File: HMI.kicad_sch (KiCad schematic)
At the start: 1 part, among them U8 XIAO-RP2350-SMD

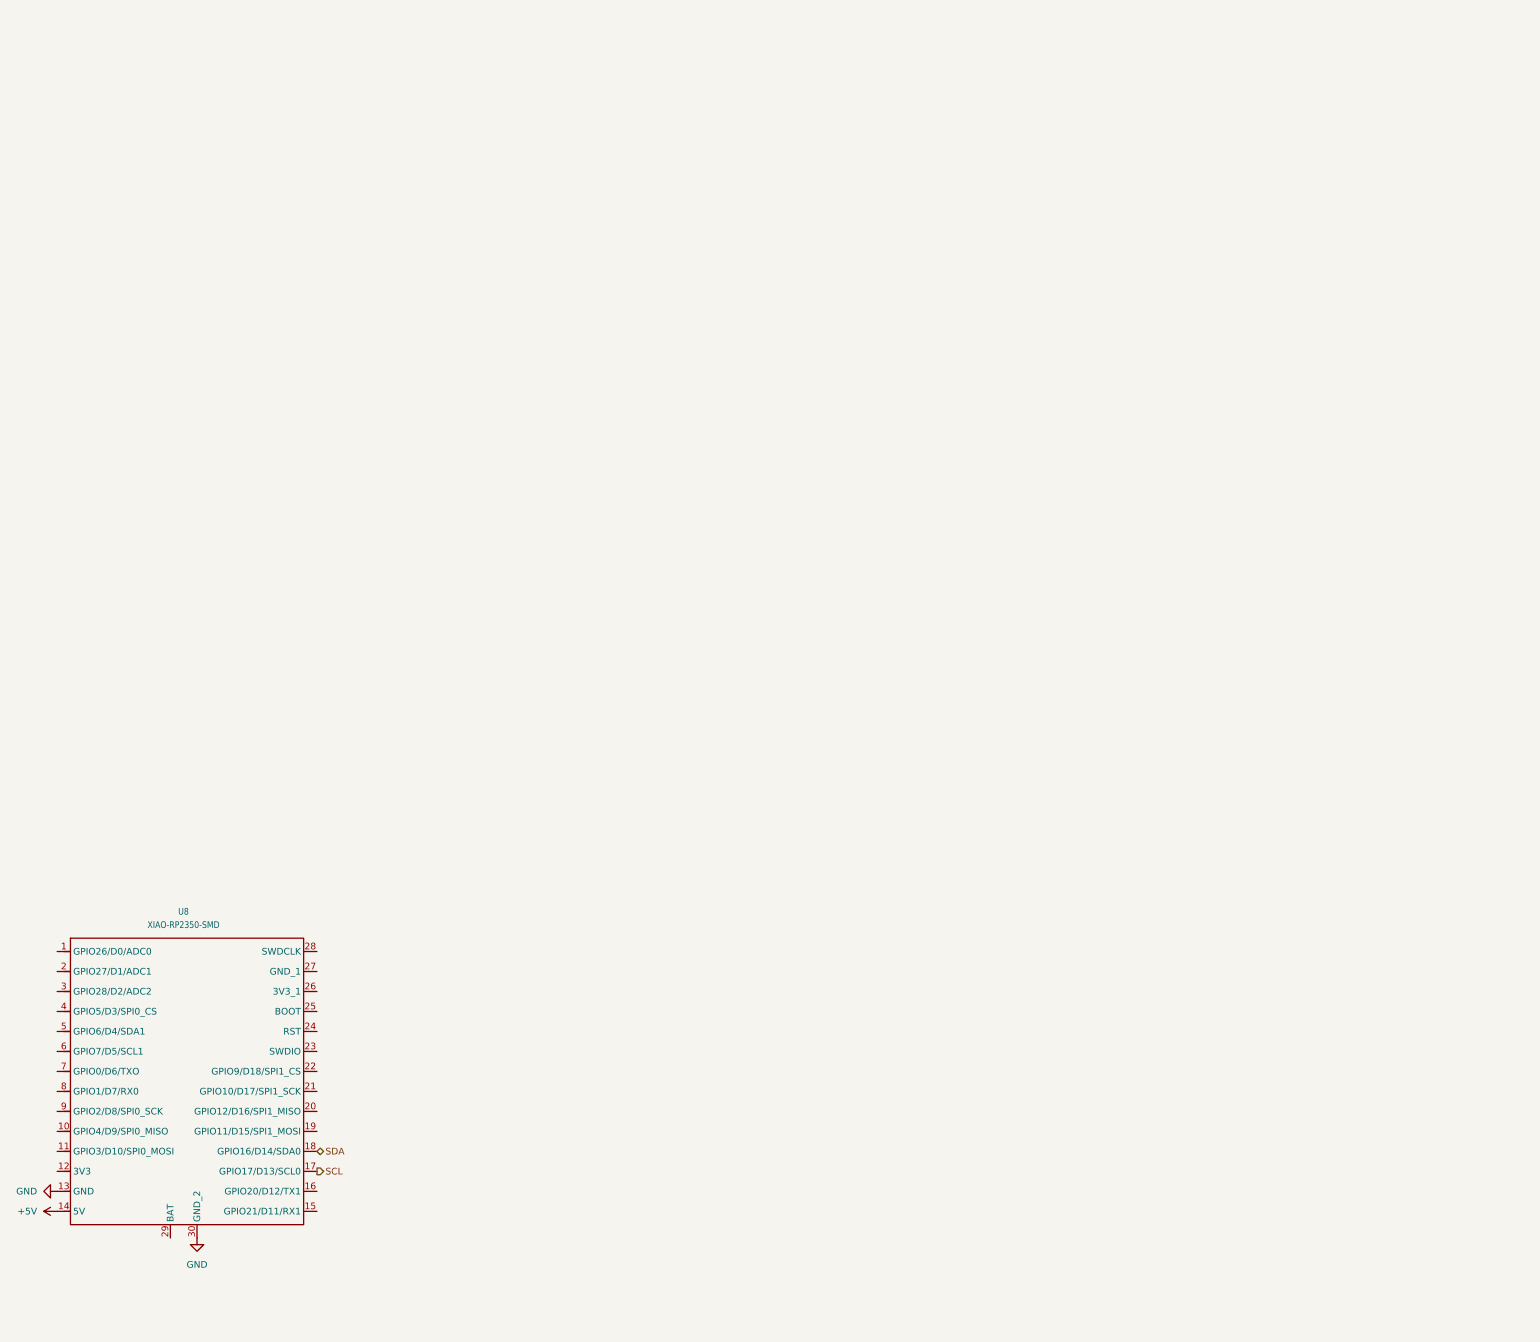
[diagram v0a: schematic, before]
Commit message: many changes
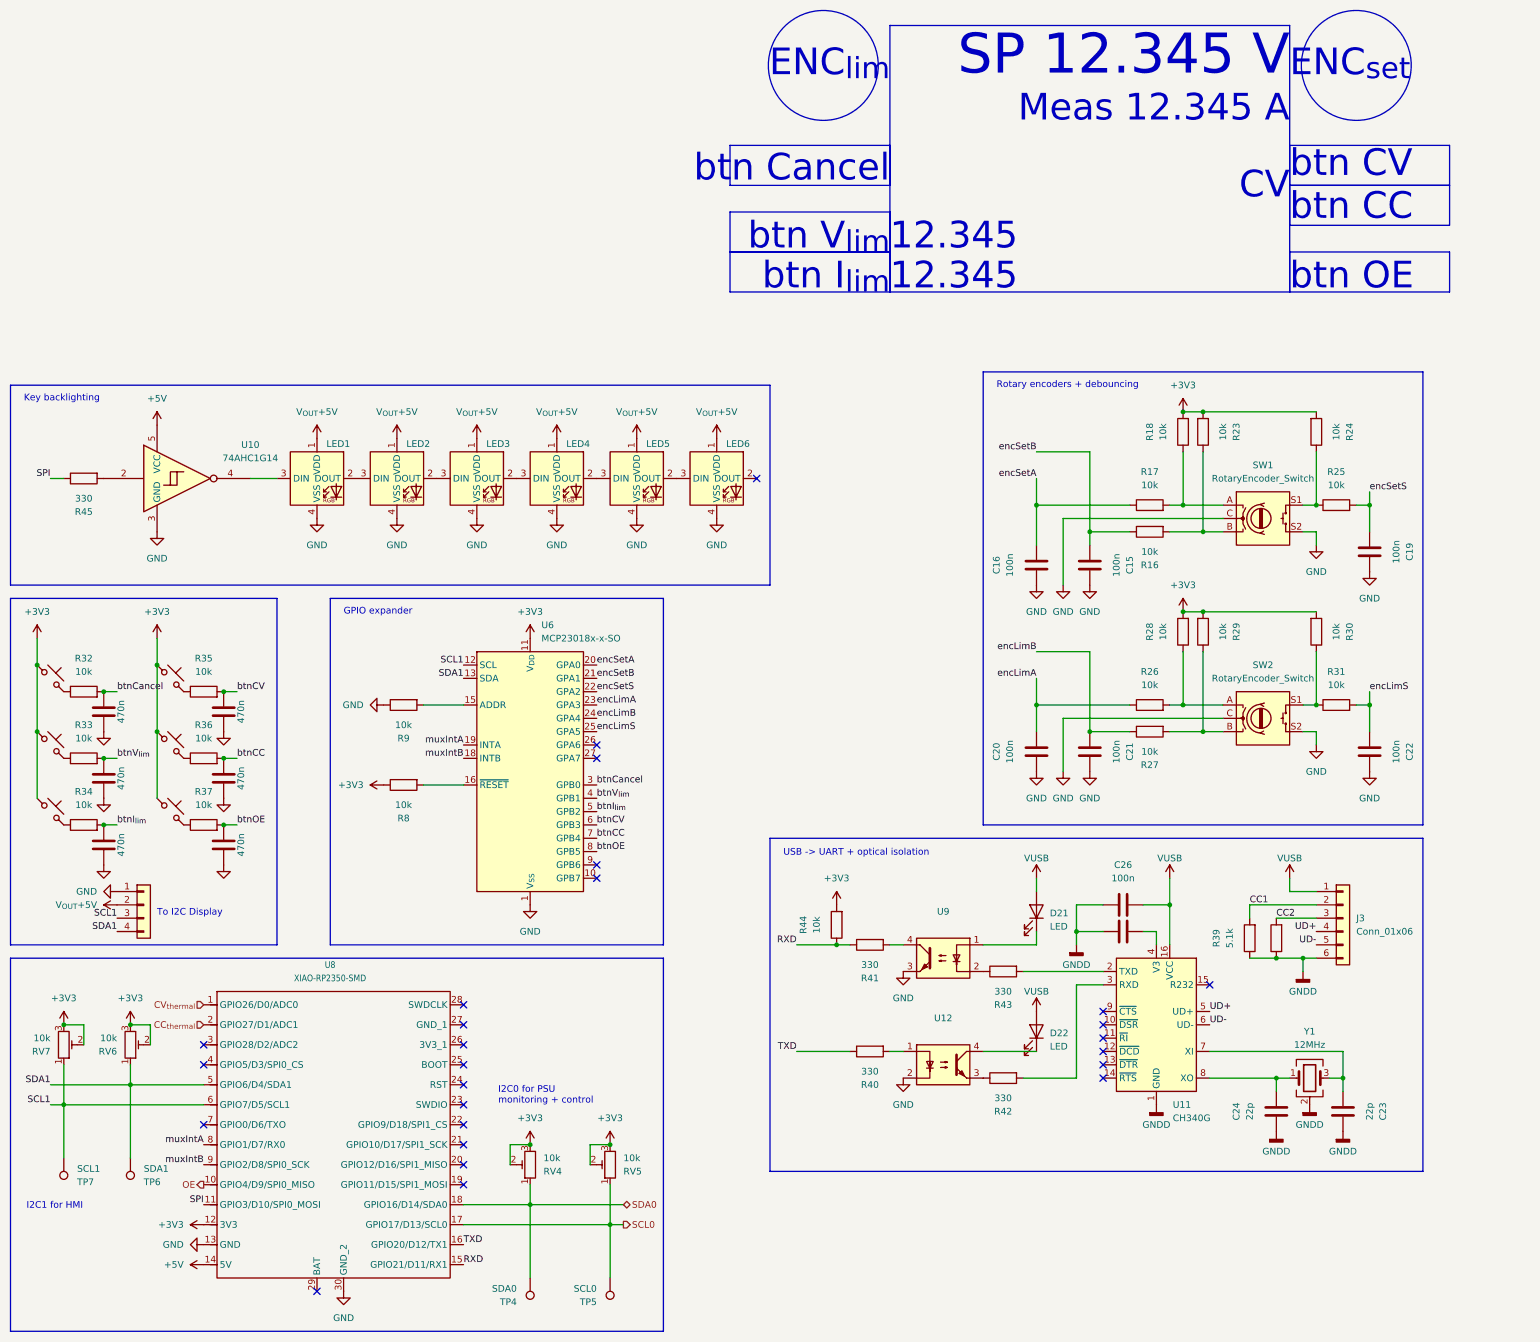
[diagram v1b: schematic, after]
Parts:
- added C12, C40, C41, C42, C43, C44: 470n, Capacitor_SMD:C_1210_3225Metric_Pad1.33x2.70mm_HandSolder, symbol Device:C
- added C15, C16, C19, C20, C21, C22, C25, C26: 100n, Capacitor_SMD:C_1210_3225Metric_Pad1.33x2.70mm_HandSolder, symbol Device:C
- added C23, C24: 22p, Capacitor_SMD:C_1210_3225Metric_Pad1.33x2.70mm_HandSolder, symbol Device:C
- added D21, D22: LED, LED_SMD:LED_1210_3225Metric_Pad1.42x2.65mm_HandSolder, symbol Device:LED
- added J2: Conn_01x04, I2C OLED:I2C OLED, symbol Connector_Generic:Conn_01x04
- added J3: Conn_01x06, Connector_JST:JST_PH_B6B-PH-K_1x06_P2.00mm_Vertical, symbol Connector_Generic:Conn_01x06
- added LED1, LED2, LED3, LED4, LED5, LED6: SK6812MINI-E, PCM_marbastlib-various:LED_6028R, symbol PCM_marbastlib-various:SK6812MINI-E
- added MX1, MX2, MX3, MX4, MX5, MX6: MX_SW_solder, PCM_marbastlib-mx:SW_MX_1u, symbol PCM_marbastlib-mx:MX_SW_solder
- added R16, R17, R18, R23, R24, R25, R26, R27, R28, R29, R30, R31, R32, R33, R34, R35, R36, R37, R44, R8, R9: 10k, Resistor_SMD:R_1210_3225Metric_Pad1.30x2.65mm_HandSolder, symbol Device:R
- added R38, R39: 5.1k, Resistor_SMD:R_1210_3225Metric_Pad1.30x2.65mm_HandSolder, symbol Device:R
- added R40, R41, R42, R43, R45: 330, Resistor_SMD:R_1210_3225Metric_Pad1.30x2.65mm_HandSolder, symbol Device:R
- added RV4, RV5, RV6, RV7: 10k, Potentiometer_THT:Potentiometer_Bourns_3299W_Vertical, symbol Device:R_Potentiometer_Trim
- added SW1, SW2: RotaryEncoder_Switch, Rotary_Encoder:RotaryEncoder_Alps_EC11E-Switch_Vertical_H20mm, symbol Device:RotaryEncoder_Switch
- added TP4: SDA0, TestPoint:TestPoint_Keystone_5019_Miniature, symbol Connector:TestPoint
- added TP5: SCL0, TestPoint:TestPoint_Keystone_5019_Miniature, symbol Connector:TestPoint
- added TP6: SDA1, TestPoint:TestPoint_Keystone_5019_Miniature, symbol Connector:TestPoint
- added TP7: SCL1, TestPoint:TestPoint_Keystone_5019_Miniature, symbol Connector:TestPoint
- added U10: 74AHC1G14, symbol 74xGxx:74AHC1G14
- added U11: CH340G, Package_SO:SOIC-16_3.9x9.9mm_P1.27mm, symbol Interface_USB:CH340G
- added U12, U9: Optocoupler_DC_PhotoNPN_AKEC, Package_DIP:DIP-4_W7.62mm_Socket_LongPads, symbol Isolator:Optocoupler_DC_PhotoNPN_AKEC
- added U6: MCP23018x-x-SO, Package_SO:SOIC-28W_7.5x17.9mm_P1.27mm, symbol Interface_Expansion:MCP23018x-x-SO
- added Y1: 12MHz, Crystal:Crystal_SMD_3225-4Pin_3.2x2.5mm, symbol Device:Crystal_GND24
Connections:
- net +5V: now also U10.5 (VCC)
- net GND: now also C12.2, C15.2, C16.2, C19.2, C20.2, C21.2, C22.2, C40.2, C41.2, C42.2, C43.2, C44.2, J2.1 (Pin_1), LED1.4 (VSS), LED2.4 (VSS), LED3.4 (VSS), LED4.4 (VSS), LED5.4 (VSS), LED6.4 (VSS), R9.1, SW1.C, SW1.S2, SW2.C, SW2.S2, U10.3 (GND), U12.2, U6.1 (V_{SS}), U9.3
- net CV_{thermal}: now reaches U8.1 (GPIO26/D0/ADC0)
- net OE: now reaches U8.10 (GPIO4/D9/SPI0_MISO)
- net SPI: now reaches U8.11 (GPIO3/D10/SPI0_MOSI)
- net SPI: now also R45.1
- net +3V3: now reaches U8.12 (3V3)
- net +3V3: now also MX1.1, MX2.1, MX3.1, MX4.1, MX5.1, MX6.1, R18.2, R23.2, R24.2, R28.2, R29.2, R30.2, R44.2, R8.1, RV4.2, RV4.3, RV5.2, RV5.3, RV6.2, RV6.3, RV7.2, RV7.3, U6.11 (V_{DD})
- net RXD: now reaches U8.15 (GPIO21/D11/RX1)
- net RXD: now also R41.1, R44.1
- net TXD: now reaches U8.16 (GPIO20/D12/TX1)
- net TXD: now also R40.1
- net CC_{thermal}: now reaches U8.2 (GPIO27/D1/ADC1)
- net SDA1: now reaches U8.5 (GPIO6/D4/SDA1)
- net SDA1: now also J2.4 (Pin_4), RV6.1, TP6.1, U6.13 (SDA)
- net SCL1: now reaches U8.6 (GPIO7/D5/SCL1)
- net SCL1: now also J2.3 (Pin_3), RV7.1, TP7.1, U6.12 (SCL)
- net muxIntA: now reaches U8.8 (GPIO1/D7/RX0)
- net muxIntA: now also U6.19 (INTA)
- net muxIntB: now reaches U8.9 (GPIO2/D8/SPI0_SCK)
- net muxIntB: now also U6.18 (INTB)
- net SCL renamed SCL0
- net SCL0: now also RV5.1, TP5.1
- net SDA renamed SDA0
- net SDA0: now also RV4.1, TP4.1
- new net: MX1.2, R32.1
- new net: MX2.2, R33.1
- new net: R16.2, R23.1, SW1.B
- new net: MX6.2, R37.1
- new net: D22.1 (K), U12.4
- new net: LED2.2 (DOUT), LED3.3 (DIN)
- new net: LED1.2 (DOUT), LED2.3 (DIN)
- new net: R26.2, R28.1, SW2.A
- new net: R30.1, R31.1, SW2.S1
- new net: LED5.2 (DOUT), LED6.3 (DIN)
- new net: LED4.2 (DOUT), LED5.3 (DIN)
- new net: LED1.3 (DIN), U10.4
- new net: R27.2, R29.1, SW2.B
- new net: R17.2, R18.1, SW1.A
- new net: C25.1, U11.4 (V3)
- new net: MX3.2, R34.1
- new net: R24.1, R25.1, SW1.S1
- new net: MX4.2, R35.1
- new net: R9.2, U6.15 (ADDR)
- new net: R8.2, U6.16 (~{RESET})
- new net: MX5.2, R36.1
- new net: R41.2, U9.4
- new net: R45.2, U10.2
- new net: D21.1 (K), U9.1
- new net: R43.1, U9.2
- new net: LED3.2 (DOUT), LED4.3 (DIN)
- new net: R43.2, U11.2 (TXD)
- new net: R42.2, U11.3 (RXD)
- new net: C23.2, U11.7 (XI), Y1.3
- new net: C24.2, U11.8 (XO), Y1.1
- new net: R40.2, U12.1
- new net: R42.1, U12.3
- new net CC1: J3.2 (Pin_2), R39.2
- new net CC2: J3.3 (Pin_3), R38.2
- new net GNDD: C23.1, C24.1, C25.2, C26.2, J3.6 (Pin_6), R38.1, R39.1, U11.1 (GND), Y1.2 (G), Y1.4 (G)
- new net UD+: J3.4 (Pin_4), U11.5 (UD+)
- new net UD-: J3.5 (Pin_5), U11.6 (UD-)
- new net VUSB: C26.1, D21.2 (A), D22.2 (A), J3.1 (Pin_1), U11.16 (VCC)
- new net V_{OUT}+5V: J2.2 (Pin_2), LED1.1 (VDD), LED2.1 (VDD), LED3.1 (VDD), LED4.1 (VDD), LED5.1 (VDD), LED6.1 (VDD)
- new net btnCC: C41.1, R36.2, U6.7 (GPB4)
- new net btnCV: C12.1, R35.2, U6.6 (GPB3)
- new net btnCancel: C42.1, R32.2, U6.3 (GPB0)
- new net btnI_{lim}: C43.1, R34.2, U6.5 (GPB2)
- new net btnOE: C44.1, R37.2, U6.8 (GPB5)
- new net btnV_{lim}: C40.1, R33.2, U6.4 (GPB1)
- new net encLimA: C20.1, R26.1, U6.23 (GPA3)
- new net encLimB: C21.1, R27.1, U6.24 (GPA4)
- new net encLimS: C22.1, R31.2, U6.25 (GPA5)
- new net encSetA: C16.1, R17.1, U6.20 (GPA0)
- new net encSetB: C15.1, R16.1, U6.21 (GPA1)
- new net encSetS: C19.1, R25.2, U6.22 (GPA2)
- no-connect marks 0 -> 26
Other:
- note added: "12.345"
- note added: "CV"
- note added: "ENC_{lim}"
- note added: "ENC_{set}"
- note added: "GPIO expander"
- note added: "I2C0 for PSU monitoring + control"
- note added: "I2C1 for HMI"
- note added: "Key backlighting"
- note added: "Meas 12.345 A"
- note added: "Rotary encoders + debouncing"
- note added: "SP 12.345 V"
- note added: "To I2C Display"
- note added: "USB -> UART + optical isolation"
- note added: "btn CV btn CC"
- note added: "btn Cancel"
- note added: "btn I_{lim}"
- note added: "btn OE"
- note added: "btn V_{lim}"
- moved on the sheet: U8
